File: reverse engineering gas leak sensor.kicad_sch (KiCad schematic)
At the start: 44 parts, among them Q1 BCX53, Q2 BCX53, Q3 BCX56, Q4 L8050QLT1G, Q5 BCX56, U3 MQ-4B, U4 NCP163ASN180T1G, U5 MC34063AG, U6 FT839NX, U7 MQ-4B

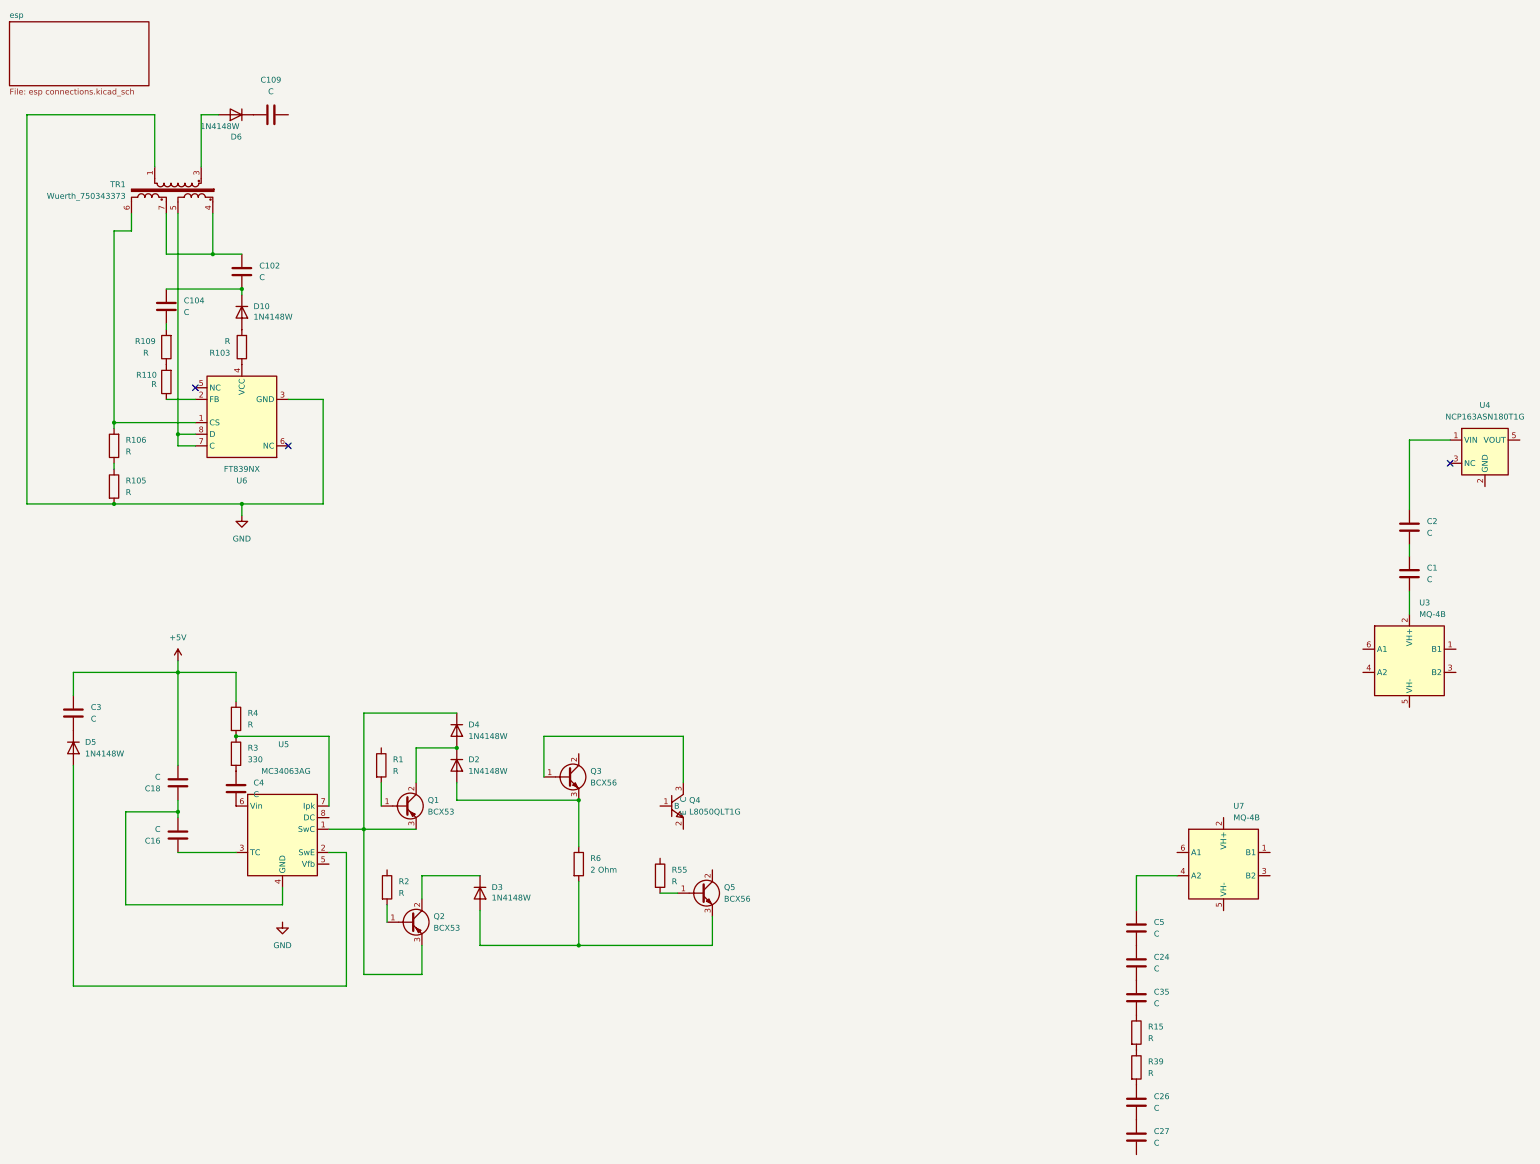
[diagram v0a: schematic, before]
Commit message: stm
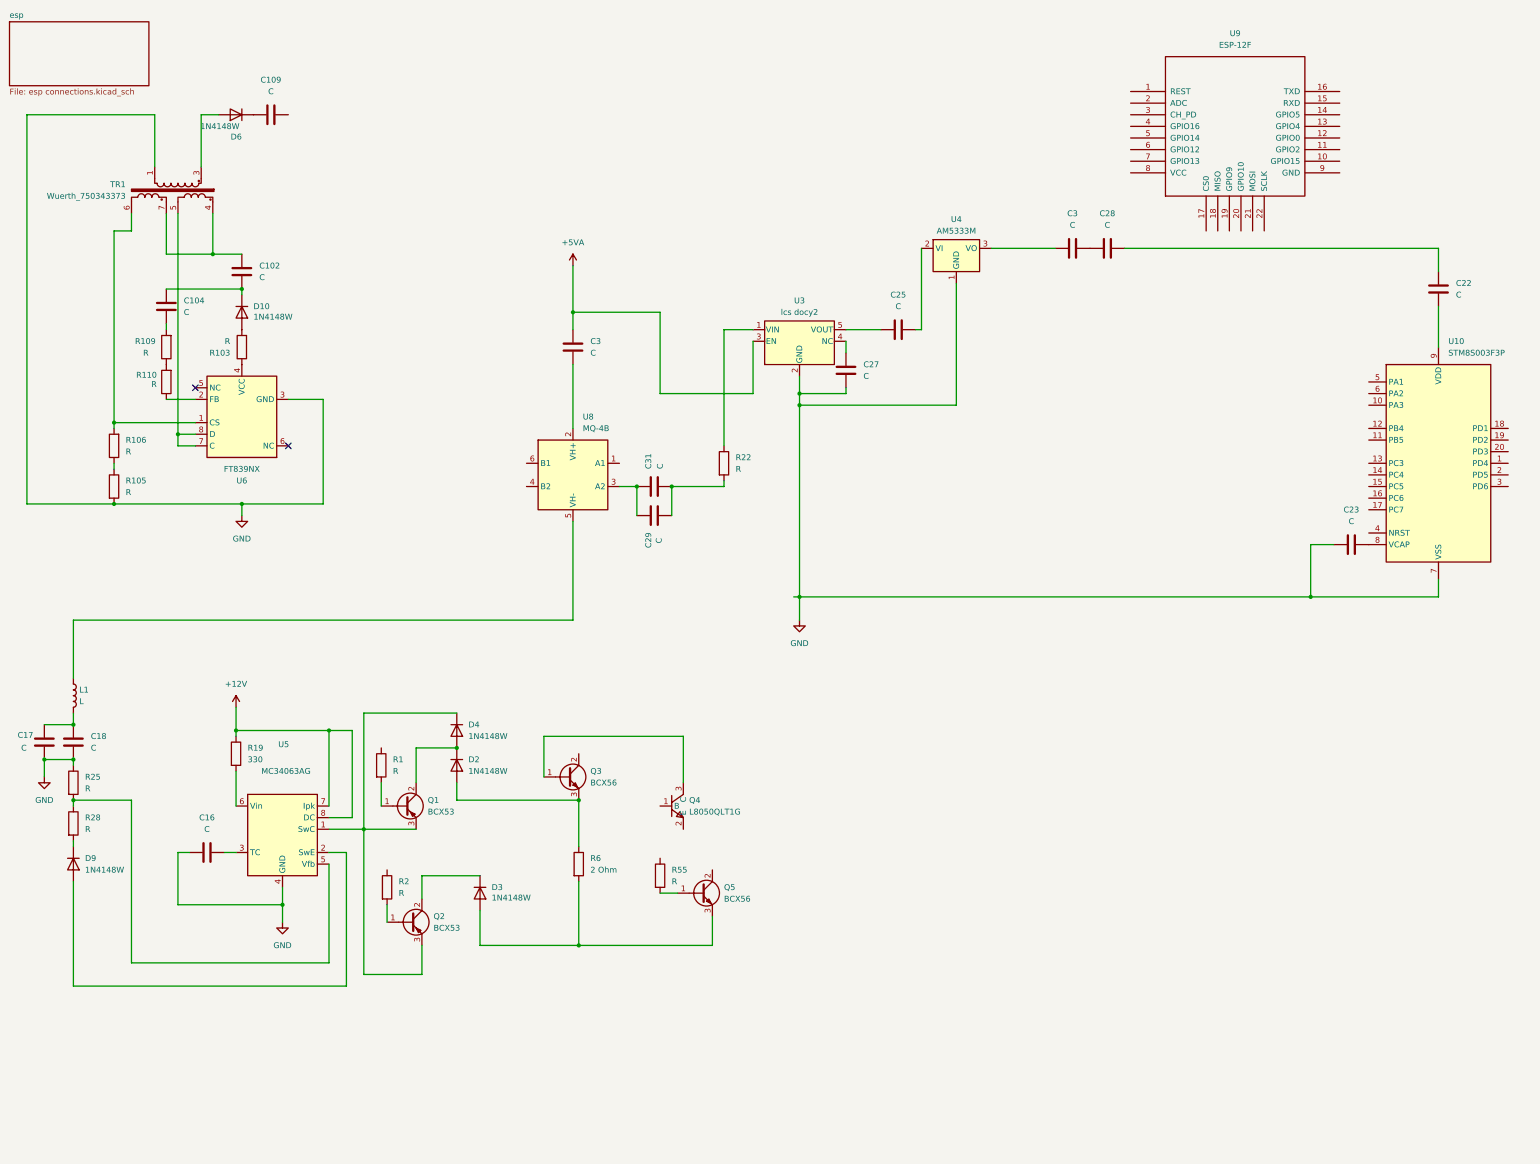
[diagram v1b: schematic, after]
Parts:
- removed C1, C18, C2, C24, C26, C35, C4, C5: C, symbol Device:C
- removed R15, R39, R4: R, symbol Device:R
- removed U3, U7: MQ-4B, Sensor:MQ-6, symbol Sensor_Gas:MQ-6
- removed U4: NCP163ASN180T1G, Package_TO_SOT_SMD:SOT-23-5, symbol Regulator_Linear:NCP163ASN180T1G
- added C17, C22, C23, C25, C28, C29, C3 (x2), C31: C, symbol Device:C
- added L1: L, symbol Device:L
- added R22, R25, R28: R, symbol Device:R
- added U10: STM8S003F3P, Package_SO:TSSOP-20_4.4x6.5mm_P0.65mm, symbol MCU_ST_STM8:STM8S003F3P
- added U3: lcs docy2, Package_TO_SOT_SMD:SOT-23-5, symbol Regulator_Linear:LP2985-1.8
- added U4: AM5333M, Photon:SOT-223-3_TabPin2, symbol Photon:U_AMS1117-3.3_SOT-223_XBLW
- added U8: MQ-4B, Sensor:MQ-6, symbol Sensor_Gas:MQ-6
- added U9: ESP-12F, symbol ESP8266:ESP-12F
- renumbered C3 to C18, D5 to D9, R3 to R19
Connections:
- net GND: now also C16.1, C18.2, C27.2, U5.4 (GND), C17.2, C23.2, R25.1, U10.7 (VSS), U3.2 (GND), U4.1 (GND)
- net +12V: now reaches R19.1, U5.7 (Ipk)
- net +12V: now also U5.8 (DC)
- net at R19.2: now also U5.6 (Vin)
- net at U5.5 (Vfb): now also R25.2, R28.1
- net at D9.1 (K): now also R28.2; no longer C18.2
- net at C27.1: now also U3.4 (NC)
- net +5V: no longer names the net of C18.1
- net +5V: now also C17.1, L1.2
- new net: C23.1, U10.8 (VCAP)
- new net: C22.1, U10.9 (VDD)
- new net: C3.2, U8.2 (VH+)
- new net: C29.1, C31.1, U8.3 (A2)
- new net: L1.1, U8.5 (VH-)
- new net: C3.1, U4.3 (VO)
- new net: C28.1, C3.2
- new net: C22.2, C28.2
- new net: R22.1, U3.1 (VIN)
- new net: C25.1, U3.5 (VOUT)
- new net: C29.2, C31.2, R22.2
- new net: C25.2, U4.2 (VI)
- new net +5VA: C3.1, U3.3 (EN)
- no-connect marks 3 -> 2
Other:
- moved on the sheet: C16, C18, D9
